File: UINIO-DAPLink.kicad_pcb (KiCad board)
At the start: 2 copper layers, 95.1 x 30 mm, 53 parts, among them J1 扩展板串口 & 电源输出, J2 扩展板 JTAG 输出, J3 JTAG_nTRST 跳线选择, J4 3.3V 跳线选择, J5 扩展板 SWD 输入, J6 DAPLink 固件下载接口, J7 SWD 下载输出, U1 ME6211C33M5G, U2 STM32F103C8T6, Y1 8MHz

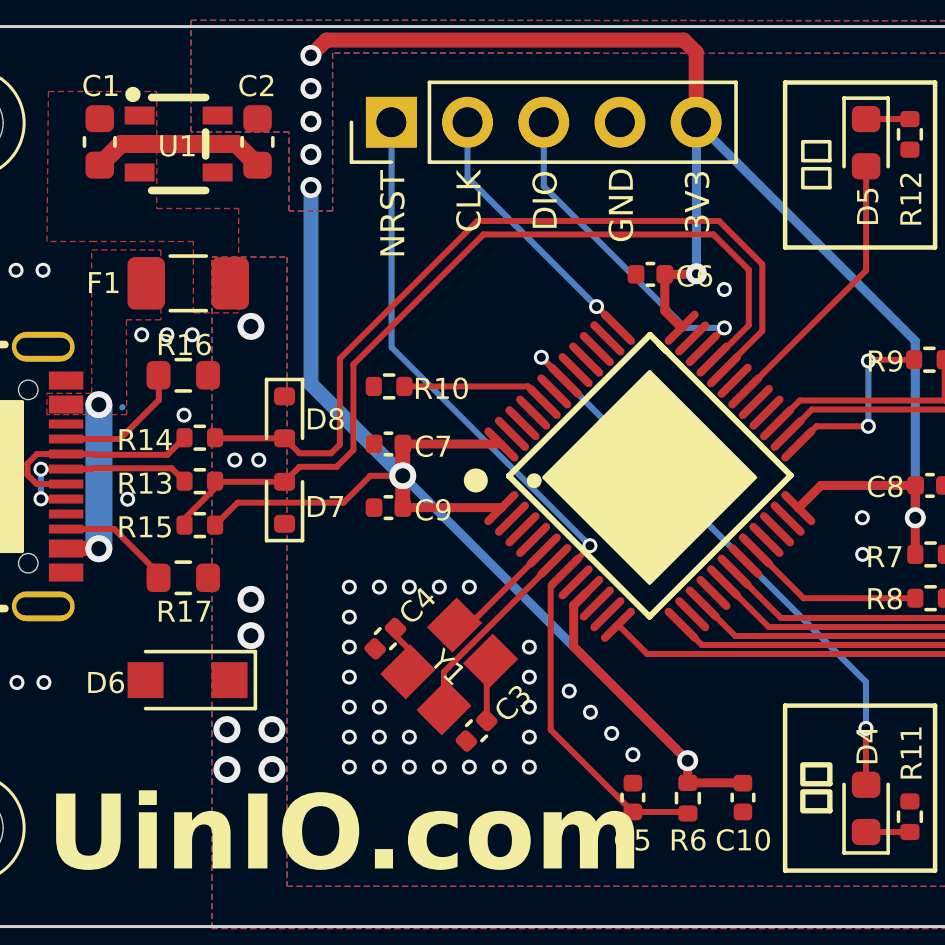
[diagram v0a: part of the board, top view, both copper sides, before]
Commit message: Release UINIO-DAPLink version 5.0.0.
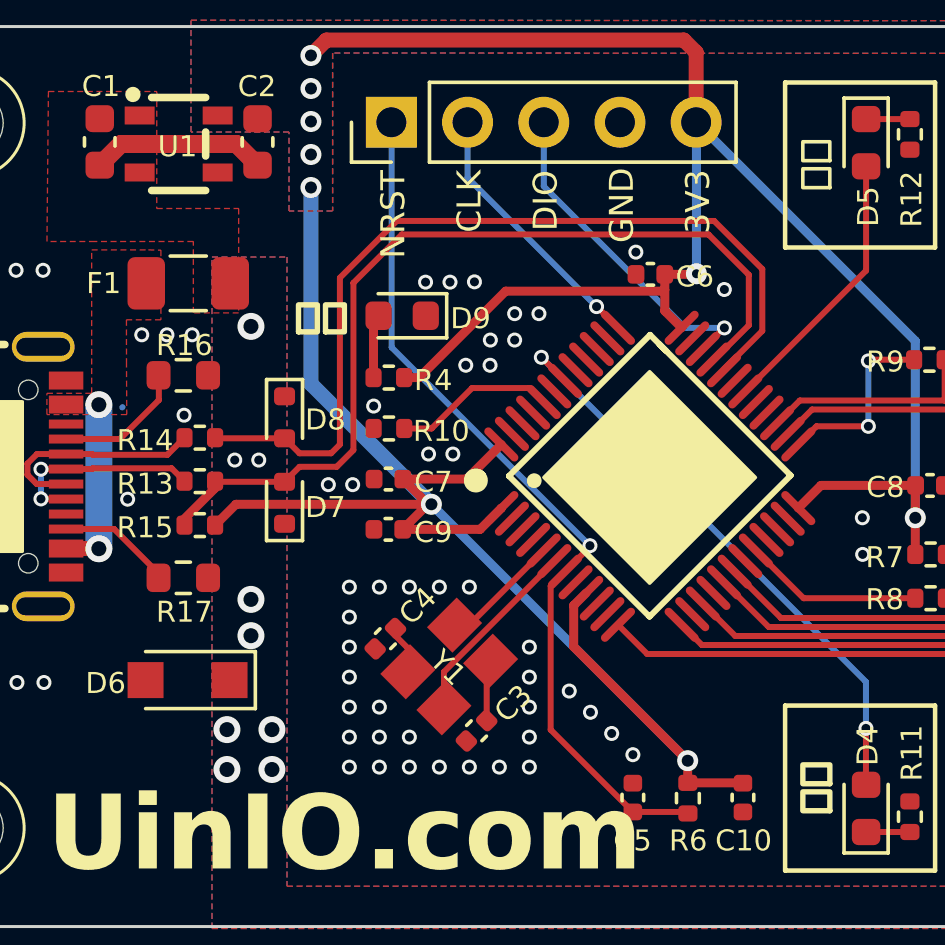
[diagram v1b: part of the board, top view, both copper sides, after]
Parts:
- added D9: LED Red, LED_SMD:LED_0603_1608Metric, F.Cu at (117.2, 97.3)
- added R4: 1K, Resistor_SMD:R_0402_1005Metric, F.Cu at (116.7, 99.3)
- moved R10 1.40 mm to (116.7, 101.0)
- moved C7 1.17 mm to (116.7, 102.7)
- moved C9 0.73 mm to (116.7, 104.4)
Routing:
- net /VDD_3.3V: track 96.0 -> 107.7 mm
- net Net-(D9-A): track 0.00 -> 1.89 mm
- net /USB_Data_P: track 28.8 -> 30.3 mm
- net /USB_Data_N: track 28.2 -> 29.7 mm
- net Net-(U2-BOOT0): track 4.86 -> 5.40 mm
- net GND: vias 66 -> 81
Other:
- board text added: "电源"
